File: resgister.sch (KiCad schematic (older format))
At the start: 6 parts, among them U1 74LS245, U2 74LS173, U3 74LS173, U4 74LS245, U5 74LS173, U6 74LS173

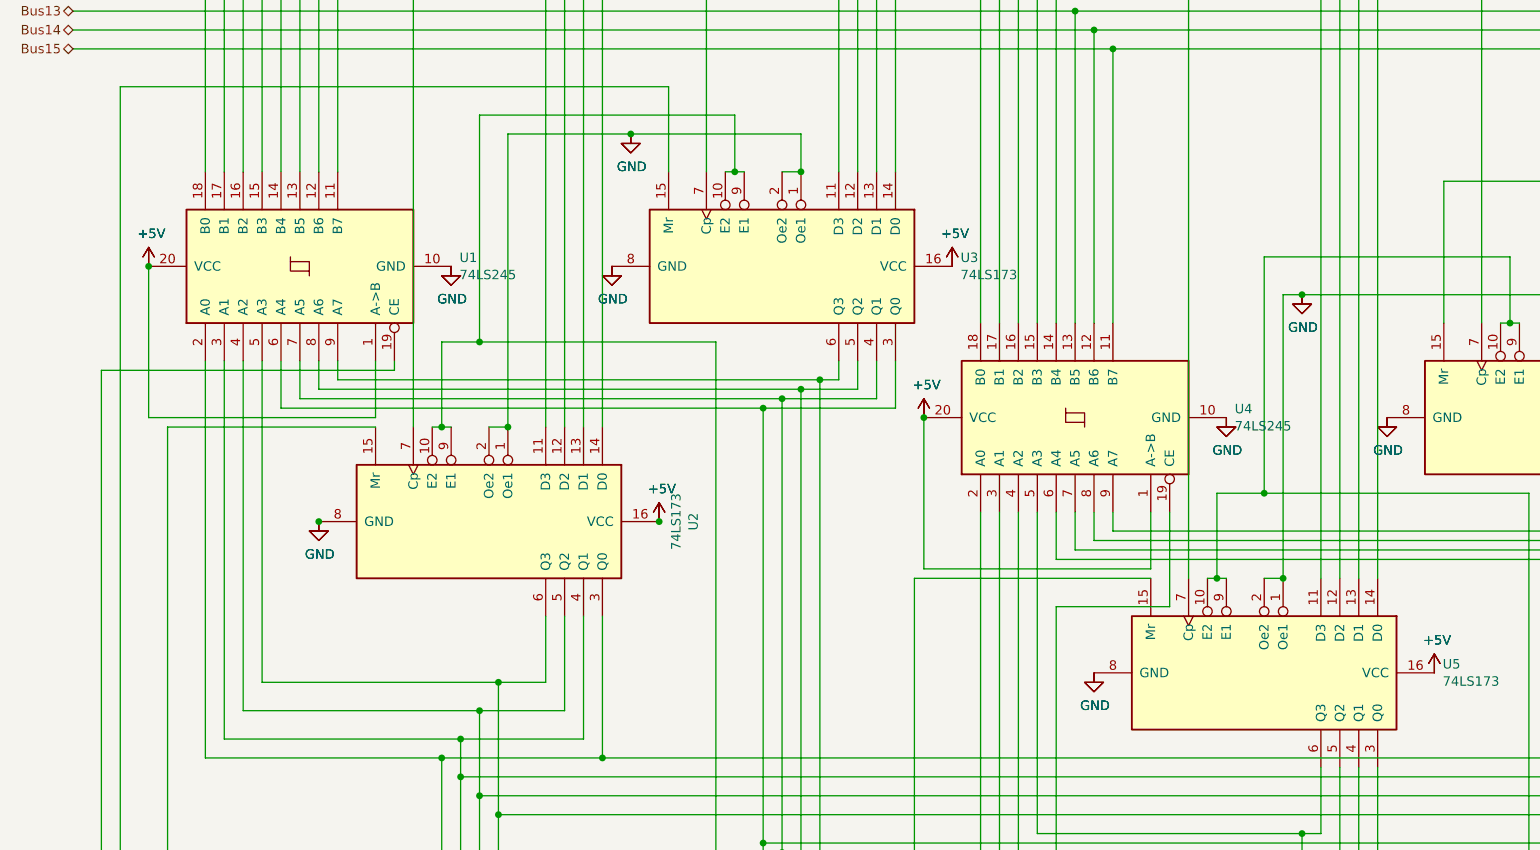
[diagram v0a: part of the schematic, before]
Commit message: fixed more errors
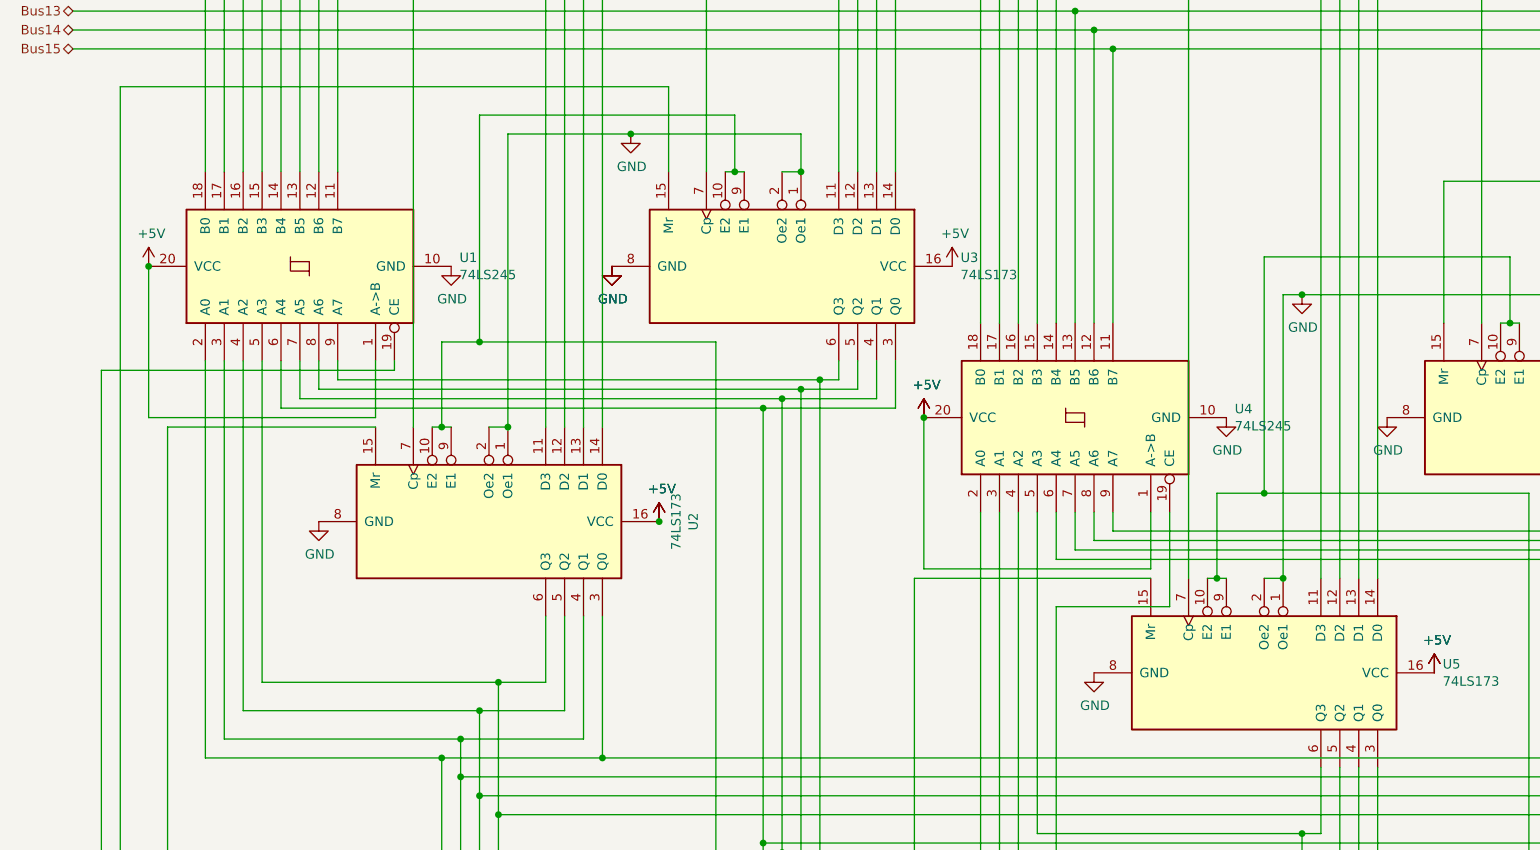
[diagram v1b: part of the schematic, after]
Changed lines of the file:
@@
-$Comp
-L 16bitCpu-rescue:GND-power #PWR?
-U 1 1 61968D2B
-P 7400 4300
-AR Path="/61968D2B" Ref="#PWR?"  Part="1"
-AR Path="/5F67C726/61968D2B" Ref="#PWR026"  Part="1"
-AR Path="/5F70885A/61968D2B" Ref="#PWR?"  Part="1"
-AR Path="/5F733C5E/61968D2B" Ref="#PWR?"  Part="1"
-AR Path="/602D4838/61968D2B" Ref="#PWR?"  Part="1"
-AR Path="/603B00C8/61968D2B" Ref="#PWR?"  Part="1"
-AR Path="/603B766D/61968D2B" Ref="#PWR?"  Part="1"
-AR Path="/5F74778C/61968D2B" Ref="#PWR055"  Part="1"
-AR Path="/5FB94562/61968D2B" Ref="#PWR?"  Part="1"
-AR Path="/616D5CDC/61968D2B" Ref="#PWR?"  Part="1"
-F 0 "#PWR055" H 7400 4050 50  0001 C CNN
-F 1 "GND" H 7405 4127 50  0000 C CNN
-F 2 "" H 7400 4300 50  0001 C CNN
-F 3 "" H 7400 4300 50  0001 C CNN
-	1    7400 4300
-	1    0    0    -1
-$EndComp
-$Comp
-L 16bitCpu-rescue:GND-power #PWR?
-U 1 1 61968D2C
-P 8250 4300
-AR Path="/61968D2C" Ref="#PWR?"  Part="1"
-AR Path="/5F67C726/61968D2C" Ref="#PWR031"  Part="1"
-AR Path="/5F70885A/61968D2C" Ref="#PWR?"  Part="1"
-AR Path="/5F733C5E/61968D2C" Ref="#PWR?"  Part="1"
-AR Path="/602D4838/61968D2C" Ref="#PWR?"  Part="1"
-AR Path="/603B00C8/61968D2C" Ref="#PWR?"  Part="1"
-AR Path="/603B766D/61968D2C" Ref="#PWR?"  Part="1"
-AR Path="/5F74778C/61968D2C" Ref="#PWR060"  Part="1"
-AR Path="/5FB94562/61968D2C" Ref="#PWR?"  Part="1"
-AR Path="/616D5CDC/61968D2C" Ref="#PWR?"  Part="1"
-F 0 "#PWR060" H 8250 4050 50  0001 C CNN
-F 1 "GND" H 8255 4127 50  0000 C CNN
-F 2 "" H 8250 4300 50  0001 C CNN
-F 3 "" H 8250 4300 50  0001 C CNN
-	1    8250 4300
-	1    0    0    -1
-$EndComp
-$Comp
-L 16bitCpu-rescue:GND-power #PWR?
-U 1 1 5F7355A3
-P 6700 5650
-AR Path="/5F7355A3" Ref="#PWR?"  Part="1"
-AR Path="/5F67C726/5F7355A3" Ref="#PWR024"  Part="1"
-AR Path="/5F70885A/5F7355A3" Ref="#PWR?"  Part="1"
-AR Path="/5F733C5E/5F7355A3" Ref="#PWR?"  Part="1"
-AR Path="/602D4838/5F7355A3" Ref="#PWR?"  Part="1"
-AR Path="/603B00C8/5F7355A3" Ref="#PWR?"  Part="1"
-AR Path="/603B766D/5F7355A3" Ref="#PWR?"  Part="1"
-AR Path="/5F74778C/5F7355A3" Ref="#PWR053"  Part="1"
-AR Path="/5FB94562/5F7355A3" Ref="#PWR?"  Part="1"
-AR Path="/616D5CDC/5F7355A3" Ref="#PWR?"  Part="1"
-F 0 "#PWR053" H 6700 5400 50  0001 C CNN
-F 1 "GND" H 6705 5477 50  0000 C CNN
-F 2 "" H 6700 5650 50  0001 C CNN
-F 3 "" H 6700 5650 50  0001 C CNN
-	1    6700 5650
-	1    0    0    -1
-$EndComp
 $Comp
 L 16bitCpu-rescue:GND-power #PWR?
@@
 	9150 3800 9250 3800
 Connection ~ 9250 3800
-$Comp
-L 16bitCpu-rescue:GND-power #PWR?
-U 1 1 6249201D
-P 7800 3650
-AR Path="/6249201D" Ref="#PWR?"  Part="1"
-AR Path="/5F67C726/6249201D" Ref="#PWR029"  Part="1"
-AR Path="/5F70885A/6249201D" Ref="#PWR?"  Part="1"
-AR Path="/5F733C5E/6249201D" Ref="#PWR?"  Part="1"
-AR Path="/602D4838/6249201D" Ref="#PWR?"  Part="1"
-AR Path="/603B00C8/6249201D" Ref="#PWR?"  Part="1"
-AR Path="/603B766D/6249201D" Ref="#PWR?"  Part="1"
-AR Path="/5F74778C/6249201D" Ref="#PWR058"  Part="1"
-AR Path="/5FB94562/6249201D" Ref="#PWR?"  Part="1"
-AR Path="/616D5CDC/6249201D" Ref="#PWR?"  Part="1"
-F 0 "#PWR058" H 7800 3400 50  0001 C CNN
-F 1 "GND" H 7805 3477 50  0000 C CNN
-F 2 "" H 7800 3650 50  0001 C CNN
-F 3 "" H 7800 3650 50  0001 C CNN
-	1    7800 3650
-	1    0    0    -1
-$EndComp
 Connection ~ 7800 3650
 Wire Wire Line
@@
 $Comp
 L 16bitCpu-rescue:GND-power #PWR?
-U 1 1 61968D2E
-P 2600 4850
-AR Path="/61968D2E" Ref="#PWR?"  Part="1"
-AR Path="/5F67C726/61968D2E" Ref="#PWR010"  Part="1"
-AR Path="/5F70885A/61968D2E" Ref="#PWR?"  Part="1"
-AR Path="/5F733C5E/61968D2E" Ref="#PWR?"  Part="1"
-AR Path="/602D4838/61968D2E" Ref="#PWR?"  Part="1"
-AR Path="/603B00C8/61968D2E" Ref="#PWR?"  Part="1"
-AR Path="/603B766D/61968D2E" Ref="#PWR?"  Part="1"
-AR Path="/5F74778C/61968D2E" Ref="#PWR039"  Part="1"
-AR Path="/5FB94562/61968D2E" Ref="#PWR?"  Part="1"
-AR Path="/616D5CDC/61968D2E" Ref="#PWR?"  Part="1"
-F 0 "#PWR039" H 2600 4600 50  0001 C CNN
-F 1 "GND" H 2605 4677 50  0000 C CNN
-F 2 "" H 2600 4850 50  0001 C CNN
-F 3 "" H 2600 4850 50  0001 C CNN
-	1    2600 4850
-	1    0    0    -1
-$EndComp
-$Comp
-L 16bitCpu-rescue:GND-power #PWR?
-U 1 1 61968D3B
-P 3300 3500
-AR Path="/61968D3B" Ref="#PWR?"  Part="1"
-AR Path="/5F67C726/61968D3B" Ref="#PWR013"  Part="1"
-AR Path="/5F70885A/61968D3B" Ref="#PWR?"  Part="1"
-AR Path="/5F733C5E/61968D3B" Ref="#PWR?"  Part="1"
-AR Path="/602D4838/61968D3B" Ref="#PWR?"  Part="1"
-AR Path="/603B00C8/61968D3B" Ref="#PWR?"  Part="1"
-AR Path="/603B766D/61968D3B" Ref="#PWR?"  Part="1"
-AR Path="/5F74778C/61968D3B" Ref="#PWR042"  Part="1"
-AR Path="/5FB94562/61968D3B" Ref="#PWR?"  Part="1"
-AR Path="/616D5CDC/61968D3B" Ref="#PWR?"  Part="1"
-F 0 "#PWR042" H 3300 3250 50  0001 C CNN
-F 1 "GND" H 3305 3327 50  0000 C CNN
-F 2 "" H 3300 3500 50  0001 C CNN
-F 3 "" H 3300 3500 50  0001 C CNN
-	1    3300 3500
-	1    0    0    -1
-$EndComp
-$Comp
-L 16bitCpu-rescue:GND-power #PWR?
 U 1 1 62492023
 P 4150 3500
@@
 $Comp
 L 16bitCpu-rescue:+5V-power #PWR?
-U 1 1 62492018
-P 1700 3500
-AR Path="/62492018" Ref="#PWR?"  Part="1"
-AR Path="/5F67C726/62492018" Ref="#PWR09"  Part="1"
-AR Path="/5F70885A/62492018" Ref="#PWR?"  Part="1"
-AR Path="/5F733C5E/62492018" Ref="#PWR?"  Part="1"
-AR Path="/602D4838/62492018" Ref="#PWR?"  Part="1"
-AR Path="/603B00C8/62492018" Ref="#PWR?"  Part="1"
-AR Path="/603B766D/62492018" Ref="#PWR?"  Part="1"
-AR Path="/5F74778C/62492018" Ref="#PWR038"  Part="1"
-AR Path="/5FB94562/62492018" Ref="#PWR?"  Part="1"
-AR Path="/616D5CDC/62492018" Ref="#PWR?"  Part="1"
-F 0 "#PWR038" H 1700 3350 50  0001 C CNN
-F 1 "+5V" H 1715 3673 50  0000 C CNN
-F 2 "" H 1700 3500 50  0001 C CNN
-F 3 "" H 1700 3500 50  0001 C CNN
-	1    1700 3500
-	1    0    0    -1
-$EndComp
-$Comp
-L 16bitCpu-rescue:+5V-power #PWR?
 U 1 1 62492019
 P 4400 4850
@@
 F 3 "" H 10050 4300 50  0001 C CNN
 	1    10050 4300
-	1    0    0    -1
-$EndComp
-$Comp
-L 16bitCpu-rescue:+5V-power #PWR?
-U 1 1 5F6AAC6B
-P 5950 3500
-AR Path="/5F6AAC6B" Ref="#PWR?"  Part="1"
-AR Path="/5F67C726/5F6AAC6B" Ref="#PWR022"  Part="1"
-AR Path="/5F70885A/5F6AAC6B" Ref="#PWR?"  Part="1"
-AR Path="/5F733C5E/5F6AAC6B" Ref="#PWR?"  Part="1"
-AR Path="/602D4838/5F6AAC6B" Ref="#PWR?"  Part="1"
-AR Path="/603B00C8/5F6AAC6B" Ref="#PWR?"  Part="1"
-AR Path="/603B766D/5F6AAC6B" Ref="#PWR?"  Part="1"
-AR Path="/5F74778C/5F6AAC6B" Ref="#PWR051"  Part="1"
-AR Path="/5FB94562/5F6AAC6B" Ref="#PWR?"  Part="1"
-AR Path="/616D5CDC/5F6AAC6B" Ref="#PWR?"  Part="1"
-F 0 "#PWR051" H 5950 3350 50  0001 C CNN
-F 1 "+5V" H 5965 3673 50  0000 C CNN
-F 2 "" H 5950 3500 50  0001 C CNN
-F 3 "" H 5950 3500 50  0001 C CNN
-	1    5950 3500
-	1    0    0    -1
-$EndComp
-$Comp
-L 16bitCpu-rescue:GND-power #PWR?
-U 1 1 61968D27
-P 4250 2800
-AR Path="/61968D27" Ref="#PWR?"  Part="1"
-AR Path="/5F67C726/61968D27" Ref="#PWR016"  Part="1"
-AR Path="/5F70885A/61968D27" Ref="#PWR?"  Part="1"
-AR Path="/5F733C5E/61968D27" Ref="#PWR?"  Part="1"
-AR Path="/602D4838/61968D27" Ref="#PWR?"  Part="1"
-AR Path="/603B00C8/61968D27" Ref="#PWR?"  Part="1"
-AR Path="/603B766D/61968D27" Ref="#PWR?"  Part="1"
-AR Path="/5F74778C/61968D27" Ref="#PWR045"  Part="1"
-AR Path="/5FB94562/61968D27" Ref="#PWR?"  Part="1"
-AR Path="/616D5CDC/61968D27" Ref="#PWR?"  Part="1"
-F 0 "#PWR045" H 4250 2550 50  0001 C CNN
-F 1 "GND" H 4255 2627 50  0000 C CNN
-F 2 "" H 4250 2800 50  0001 C CNN
-F 3 "" H 4250 2800 50  0001 C CNN
-	1    4250 2800
 	1    0    0    -1
 $EndComp
@@
 Connection ~ 3600 4350
 Connection ~ 4400 4850
-Connection ~ 2600 4850
 Wire Wire Line
 	10250 3050 10250 7750
